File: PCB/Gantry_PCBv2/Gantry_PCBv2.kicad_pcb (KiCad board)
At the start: 2 copper layers, 120 x 120 mm, 64 parts, among them J1 Conn_01x14, J10 B2B-XH-A_LF__SN_, J11 B2B-XH-A_LF__SN_, J12 B2B-XH-A_LF__SN_, J13 Conn_01x03_Pin, J14 USB_C_Receptacle_USB2.0_16P, J17 B2B-XH-A_LF__SN_, J2 Conn_01x14, J3 Conn_01x10, J4 Screw_Terminal_01x02, J5 DCJ200-10-A-XX-X_REVA, J6 Conn_01x04_Pin, J7 Conn_01x04_Pin, J8 Conn_01x04_Pin, J9 Conn_01x04_Pin, Q1 SS8050, Q2 SS8050, SW7 SW_0, SW8 SW_EN, U1 ESP32-WROOM-32E, U2 CH340C, U3 TB6612FNG H-bridge Motor Driv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, U4 LM2576S-5, U5 AMS1117-3.3, U6 DRV8825_STEPPER_MOTOR_DRIVER_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, U7 DRV8825_STEPPER_MOTOR_DRIVER_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, U8 DRV8825_STEPPER_MOTOR_DRIVER_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, U9 DRV8825_STEPPER_MOTOR_DRIVER_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

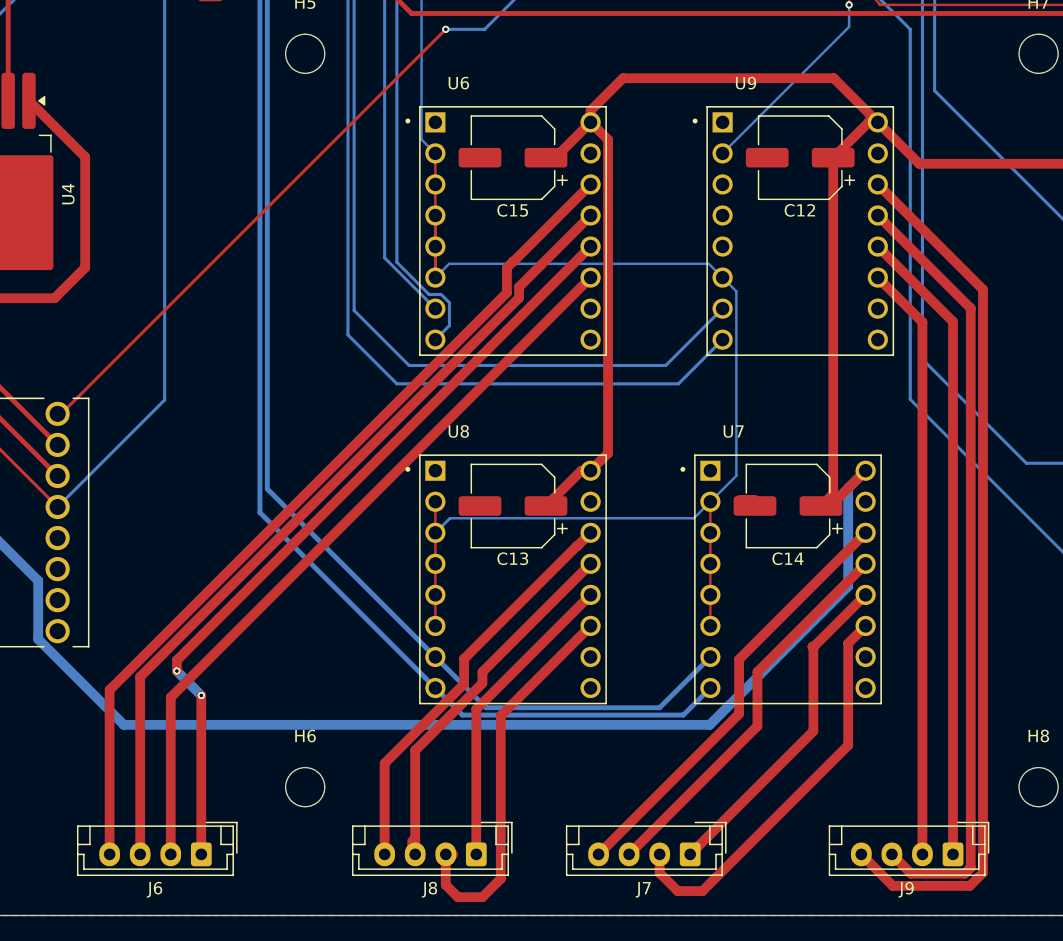
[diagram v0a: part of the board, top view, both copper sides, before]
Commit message: Schematic v3
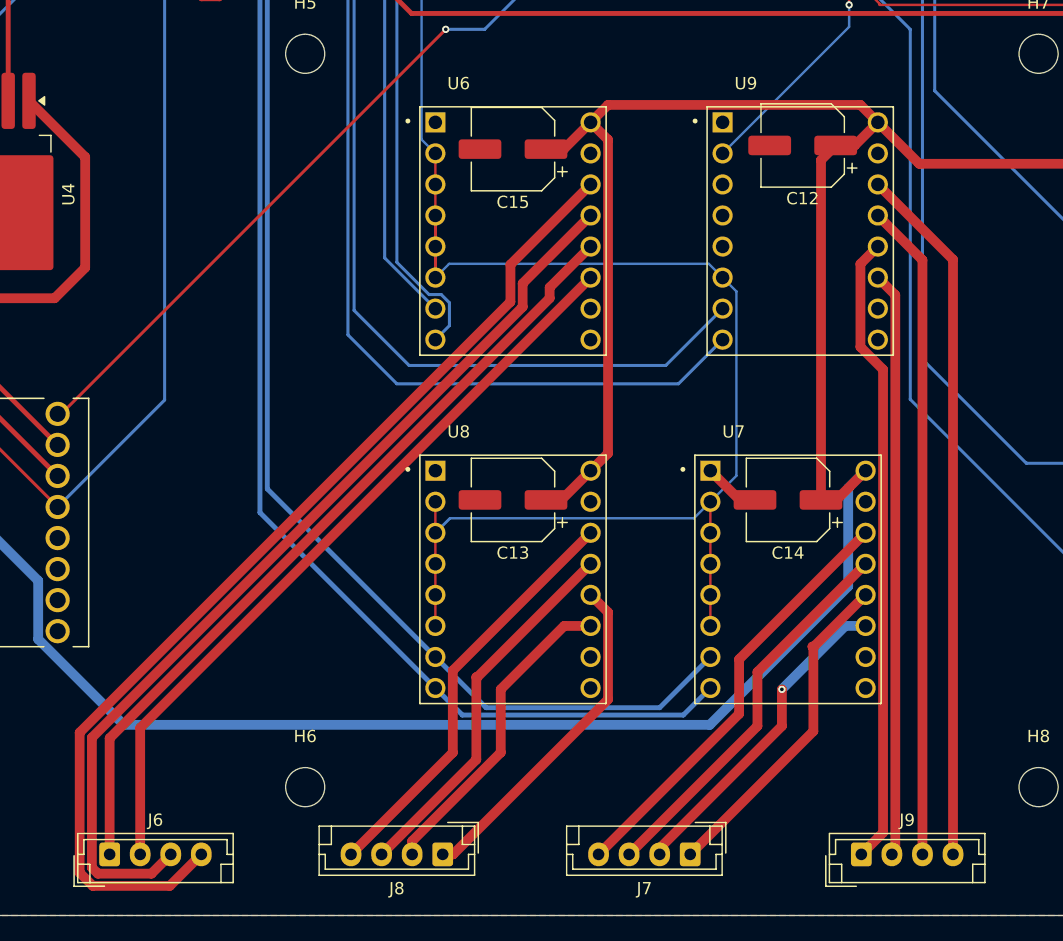
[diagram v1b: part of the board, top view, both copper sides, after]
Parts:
- moved J6 7.50 mm to (82.5, 165.0), turned to 0 degrees
- moved J9 7.50 mm to (144.0, 165.0), turned to 0 degrees
- moved J8 2.75 mm to (109.8, 165.0)
- moved C12 1.02 mm to (139.2, 107.0)
- moved C15 0.70 mm to (115.5, 107.3)
- moved C13 0.50 mm to (115.5, 136.0)
- moved C14 0.50 mm to (138.0, 136.0)
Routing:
- net /SM1_B2: track 71.3 -> 57.4 mm
- net /SM2_B2: track 71.1 -> 85.1 mm
- net /SM1_B1: track 64.2 -> 53.8 mm
- net /SM2_B1: track 67.5 -> 77.6 mm
- net /SM3_A2: track 33.4 -> 26.6 mm, vias 0 -> 1
- net /SM4_A2: track 32.6 -> 26.0 mm
- net GND: track 20.1 -> 23.5 mm
- net /12V_P: track 234.1 -> 231.0 mm
- net /SM4_A1: track 25.1 -> 27.9 mm
- net /SM2_A1: track 64.6 -> 66.0 mm, vias 2 -> 0
- net /SM4_B2: track 33.3 -> 34.4 mm
- net /SM2_A2: track 61.4 -> 62.5 mm
- net /SM1_A2: track 48.7 -> 47.9 mm
